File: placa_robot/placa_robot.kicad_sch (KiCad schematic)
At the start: 1 part, among them IC1 MSP430FR2355TPT

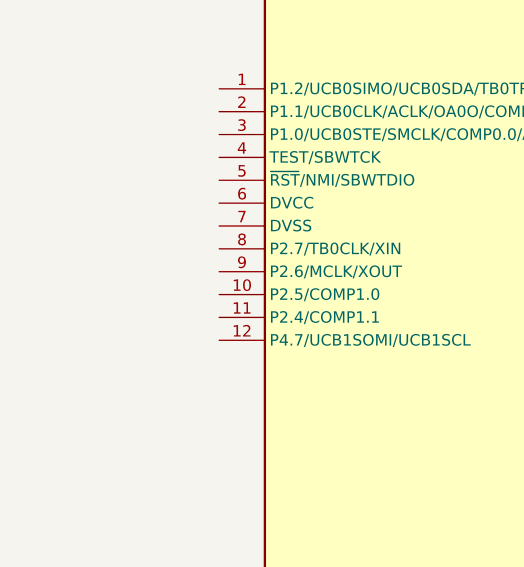
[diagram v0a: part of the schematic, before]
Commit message: merge
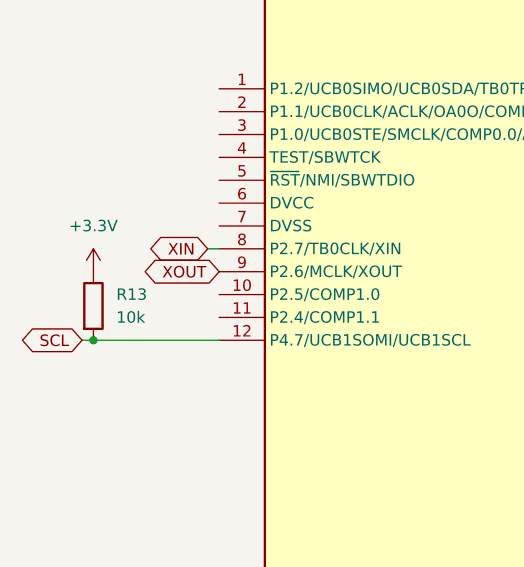
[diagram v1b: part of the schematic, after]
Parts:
- added R13: 10k, symbol Device:R
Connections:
- net SCL: now reaches IC1.12 (P4.7/UCB1SOMI/UCB1SCL)
- net SCL: now also R13.2
- net XIN: now reaches IC1.8 (P2.7/TB0CLK/XIN)
- net XOUT: now reaches IC1.9 (P2.6/MCLK/XOUT)
- new net +3.3V: R13.1
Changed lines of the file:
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@@
+		)
+	)
+	(junction
+		(at 124.46 152.4)
+		(diameter 0)
+		(color 0 0 0 0)
+	)
+	(wire
+		(pts
+			(xy 137.16 142.24) (xy 138.43 142.24)
+		)
+		(stroke
+			(width 0)
+			(type default)
+		)
+	)
+	(wire
+		(pts
+			(xy 124.46 152.4) (xy 138.43 152.4)
+		)
+		(stroke
+			(width 0)
+			(type default)
+		)
+	)
+	(wire
+		(pts
+			(xy 123.19 152.4) (xy 124.46 152.4)
+		)
+		(stroke
+			(width 0)
+			(type default)
+		)
+	)
+	(global_label "XIN"
+		(shape bidirectional)
+		(at 137.16 142.24 180)
+		(fields_autoplaced yes)
+		(effects
+			(font
+				(size 1.27 1.27)
+			)
+			(justify right)
+		)
+		(property "Intersheetrefs" "${INTERSHEET_REFS}"
+			(at 129.9187 142.24 0)
+			(effects
+				(font
+					(size 1.27 1.27)
+				)
+				(justify right)
+				(hide yes)
+			)
+		)
+	)
+	(global_label "XOUT"
+		(shape bidirectional)
+		(at 138.43 144.78 180)
+		(fields_autoplaced yes)
+		(effects
+			(font
+				(size 1.27 1.27)
+			)
+			(justify right)
+		)
+		(property "Intersheetrefs" "${INTERSHEET_REFS}"
+			(at 129.4954 144.78 0)
+			(effects
+				(font
+					(size 1.27 1.27)
+				)
+				(justify right)
+				(hide yes)
+			)
 		)
 	)
@@
 		)
 	)
+	(global_label "SCL"
+		(shape bidirectional)
+		(at 123.19 152.4 180)
+		(fields_autoplaced yes)
+		(effects
+			(font
+				(size 1.27 1.27)
+			)
+			(justify right)
+		)
+		(property "Intersheetrefs" "${INTERSHEET_REFS}"
+			(at 115.5859 152.4 0)
+			(effects
+				(font
+					(size 1.27 1.27)
+				)
+				(justify right)
+				(hide yes)
+			)
+		)
+	)
 	(global_label "Joystick_Boton"
 		(shape input)
@@
 				(justify left)
 				(hide yes)
+			)
+		)
+	)
+	(symbol
+		(lib_id "Device:R")
+		(at 124.46 148.59 0)
+		(unit 1)
+		(exclude_from_sim no)
+		(in_bom yes)
+		(on_board yes)
+		(dnp no)
+		(fields_autoplaced yes)
+		(property "Reference" "R13"
+			(at 127 147.3199 0)
+			(effects
+				(font
+					(size 1.27 1.27)
+				)
+				(justify left)
+			)
+		)
+		(property "Value" "10k"
+			(at 127 149.8599 0)
+			(effects
+				(font
+					(size 1.27 1.27)
+				)
+				(justify left)
+			)
+		)
+		(property "Footprint" ""
+			(at 122.682 148.59 90)
+			(effects
+				(font
+					(size 1.27 1.27)
+				)
+				(hide yes)
+			)
+		)
+		(property "Datasheet" "~"
+			(at 124.46 148.59 0)
+			(effects
+				(font
+					(size 1.27 1.27)
+				)
+				(hide yes)
+			)
+		)
+		(property "Description" "Resistor"
+			(at 124.46 148.59 0)
+			(effects
+				(font
+					(size 1.27 1.27)
+				)
+				(hide yes)
+			)
+		)
+		(pin "2"
+		)
+		(pin "1"
+		)
+		(instances
+			(project "placa_robot"
+				(path "/8aa50d15-d96a-41b3-aa5f-664bff39212d"
+					(reference "R13")
+					(unit 1)
+				)
 			)
 		)
@@
 					(unit 1)
 				)
+			)
+		)
+	)
+	(symbol
+		(lib_id "power:+3.3V")
+		(at 124.46 144.78 0)
+		(unit 1)
+		(exclude_from_sim no)
+		(in_bom yes)
+		(on_board yes)
+		(dnp no)
+		(fields_autoplaced yes)
+		(property "Reference" "#PWR011"
+			(at 124.46 148.59 0)
+			(effects
+				(font
+					(size 1.27 1.27)
+				)
+				(hide yes)
+			)
+		)
+		(property "Value" "+3.3V"
+			(at 124.46 139.7 0)
+			(effects
+				(font
+					(size 1.27 1.27)
+				)
+			)
+		)
+		(property "Footprint" ""
+			(at 124.46 144.78 0)
+			(effects
+				(font
+					(size 1.27 1.27)
+				)
+				(hide yes)
+			)
+		)
+		(property "Datasheet" ""
+			(at 124.46 144.78 0)
+			(effects
+				(font
+					(size 1.27 1.27)
+				)
+				(hide yes)
+			)
+		)
+		(property "Description" "Power symbol creates a global label with name \"+3.3V\""
+			(at 124.46 144.78 0)
+			(effects
+				(font
+					(size 1.27 1.27)
+				)
+				(hide yes)
+			)
+		)
+		(pin "1"
+		)
+		(instances
+			(project "placa_robot"
+				(path "/8aa50d15-d96a-41b3-aa5f-664bff39212d"
+					(reference "#PWR011")
+					(unit 1)
+				)

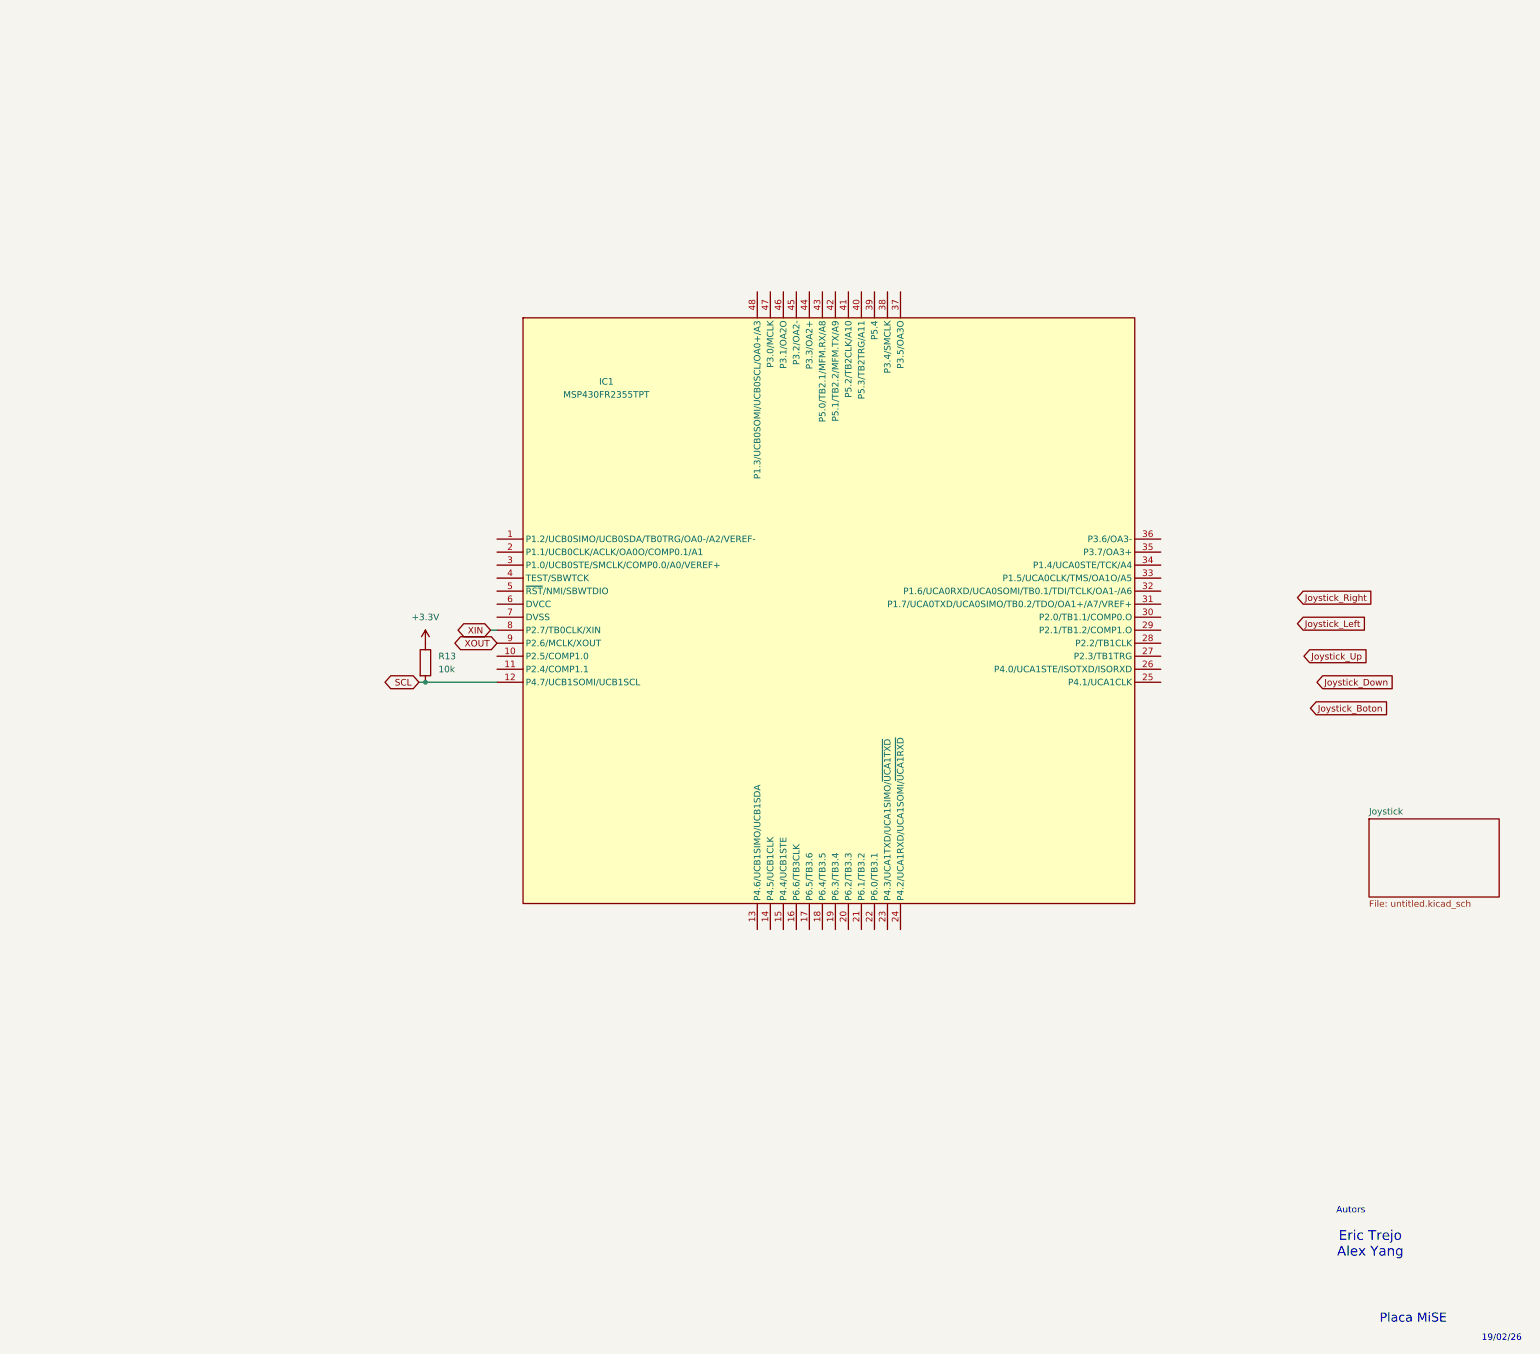
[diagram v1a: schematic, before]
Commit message: Fotoresistores
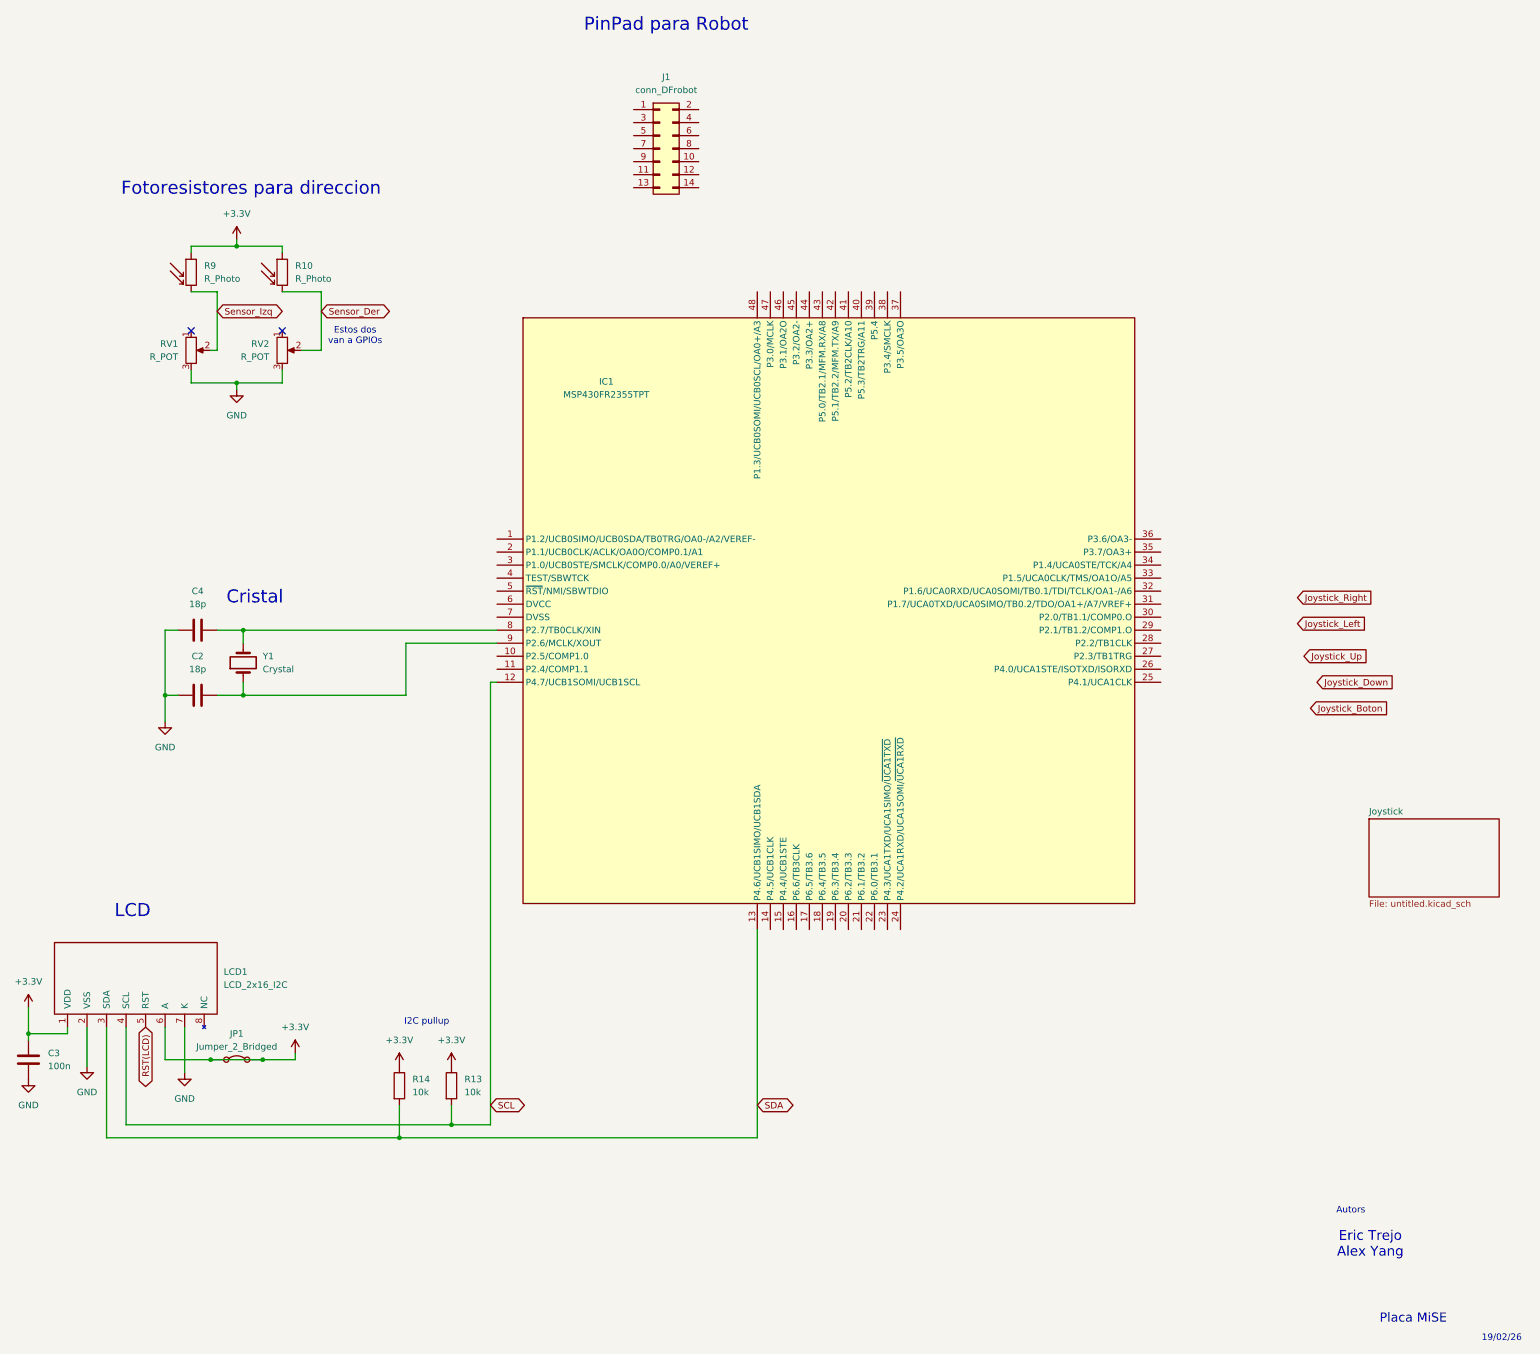
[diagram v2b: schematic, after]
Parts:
- added C2, C4: 18p, symbol Device:C
- added C3: 100n, symbol Device:C
- added J1: conn_DFrobot, MiSE:conn_DFrobot, symbol MiSE:conn_DFrobot
- added JP1: Jumper_2_Bridged, symbol Jumper:Jumper_2_Bridged
- added LCD1: LCD_2x16_I2C, symbol MiSE:LCD_2x16_I2C
- added R10, R9: R_Photo, symbol Device:R_Photo
- added R14: 10k, symbol Device:R
- added RV1, RV2: R_POT, MiSE:Trimmer_MiSE, symbol MiSE:R_POT-Device
- added Y1: Crystal, Crystal:Crystal_DS26_D2.0mm_L6.0mm_Horizontal, symbol Device:Crystal
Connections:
- net +3.3V: now also C3.1, JP1.1 (A), JP1.2 (B), LCD1.1 (VDD), LCD1.6 (A), R10.1, R14.1, R9.1
- net SCL: now also LCD1.4 (SCL)
- net SDA: now reaches IC1.13 (P4.6/UCB1SIMO/UCB1SDA)
- net SDA: now also LCD1.3 (SDA), R14.2
- net XIN: no longer names the net of IC1.8 (P2.7/TB0CLK/XIN)
- net XIN: now also C4.2, Y1.2
- net XOUT: no longer names the net of IC1.9 (P2.6/MCLK/XOUT)
- net XOUT: now also C2.2, Y1.1
- new net GND: C2.1, C3.2, C4.1, LCD1.2 (VSS), LCD1.7 (K), RV1.3, RV2.3
- new net RST(LCD): LCD1.5 (RST)
- new net Sensor_Der: R10.2, RV2.2
- new net Sensor_Izq: R9.2, RV1.2
- no-connect marks 0 -> 2
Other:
- note added: "Cristal"
- note added: "Estos dos van a GPIOs"
- note added: "Fotoresistores para direccion"
- note added: "I2C pullup"
- note added: "LCD"
- note added: "PinPad para Robot"
- moved on the sheet: R13
